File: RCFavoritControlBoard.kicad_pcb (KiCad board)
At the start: 2 copper layers, 30 parts, among them J3 Conn_01x03_Pin, U1 SY8303, U2 TPS7A20xxxPDBVR, U3 DRV8833PWP

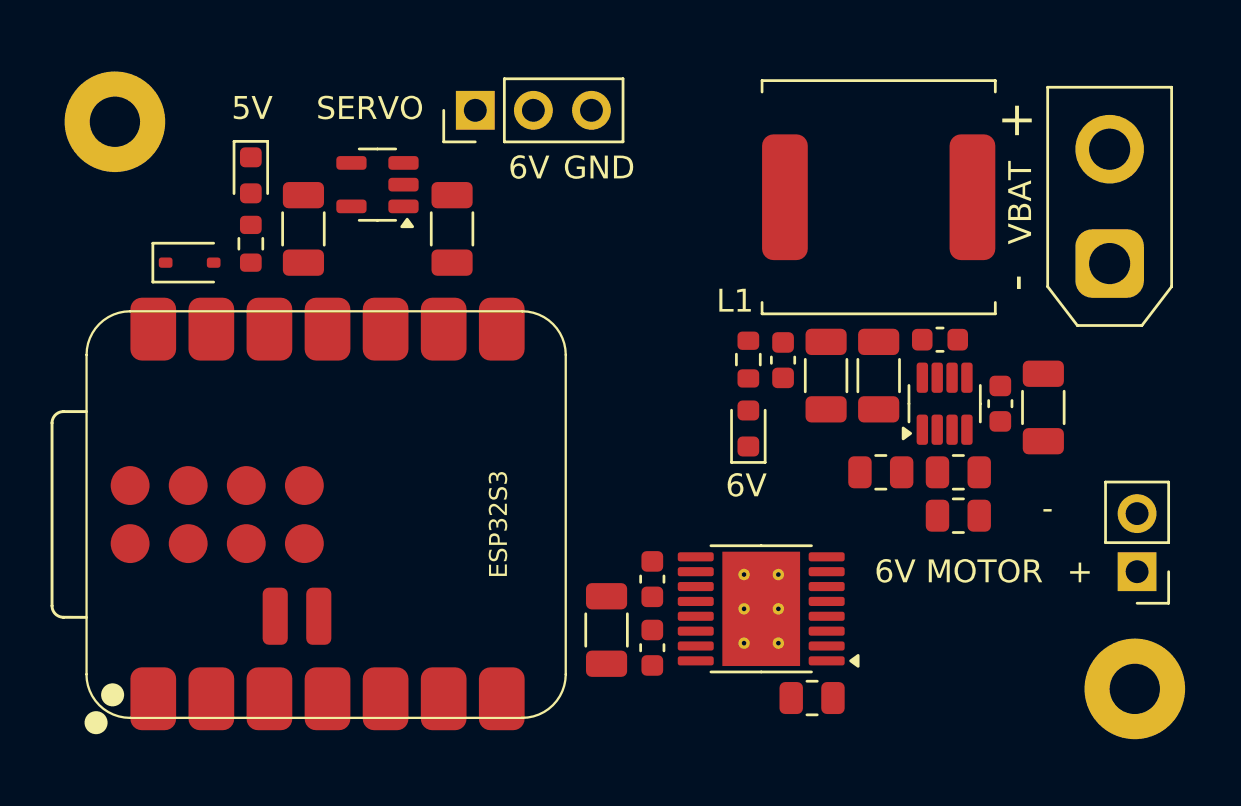
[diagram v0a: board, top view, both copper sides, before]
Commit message: routing done
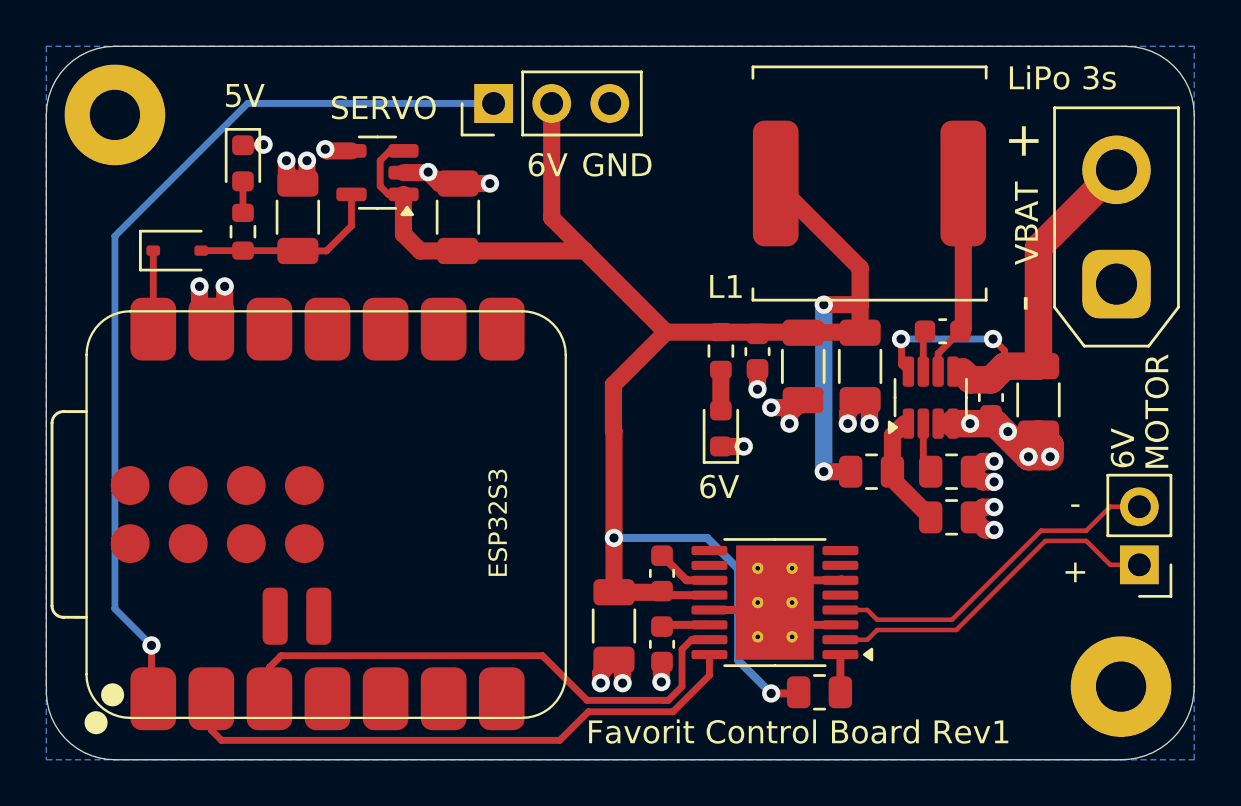
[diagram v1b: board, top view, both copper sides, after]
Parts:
- MOTOR: renamed from 6V MOTOR
- moved R2 1.26 mm to (151.5, 89.3)
- moved D1 1.20 mm to (151.5, 92.7)
- moved C6 1.18 mm to (153.1, 89.3)
- moved C4 1.08 mm to (155.1, 90.0)
- moved VBAT 0.95 mm to (168.8, 86.4)
- moved C5 0.91 mm to (157.6, 90.0)
- moved J3 0.85 mm to (141.6, 78.5)
- moved D3 0.76 mm to (127.7, 84.9)
- moved L1 0.72 mm to (158.0, 82.0)
- moved U1 0.66 mm to (160.7, 91.4)
- moved U3 0.66 mm to (153.9, 100.3)
- moved 5V 0.63 mm to (130.6, 81.1)
- moved R5 0.63 mm to (130.6, 84.1)
- moved H1 0.61 mm to (169.0, 104.0)
- moved C8 0.57 mm to (140.0, 83.5)
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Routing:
- net +6V: track 0.00 -> 82.0 mm, vias 0 -> 4
- net GND: track 0.00 -> 43.3 mm, vias 0 -> 25
- net SERVO_PWM: track 0.00 -> 39.9 mm, vias 0 -> 1
- net DRV8833_IN1: track 0.00 -> 25.4 mm
- net DRV8833_IN2: track 0.00 -> 23.7 mm
- net VBAT: track 0.00 -> 20.7 mm, vias 0 -> 2
- net Motor+: track 0.00 -> 15.3 mm
- net Motor-: track 0.00 -> 15.3 mm
- net Net-(U1-LX): track 0.00 -> 8.68 mm
- net +5V: track 0.00 -> 8.41 mm
- net Net-(U1-FB): track 0.00 -> 5.01 mm
- net Net-(D3-K): track 0.00 -> 3.43 mm
- net Net-(U3-VCP): track 0.00 -> 2.52 mm
- net Net-(U1-FS): track 0.00 -> 2.24 mm
- net Net-(U3-VINT): track 0.00 -> 2.11 mm
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- added copper zone on B.Cu, net GND
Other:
- board outline added: 50.2 x 31.2 mm
- board text added: "Favorit Control Board Rev1"
- board text added: "LiPo 3s"
